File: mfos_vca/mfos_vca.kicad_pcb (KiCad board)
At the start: 2 copper layers, 196.4 x 297.5 mm, 95 parts, among them J1 CV A, J2 Signal In A, J3 Signal Out A, J4 CV B, J5 CV1 B, J5 Signal In B, J6 Signal Out B, J7 Conn_02x05_Odd_Even, Q1 2N3904, Q2 2N3906, Q3 2N3904, Q4 2N3906, SW1 SW_SPDT, SW2 SW_SPDT, U1 TL074, U2 LM13700

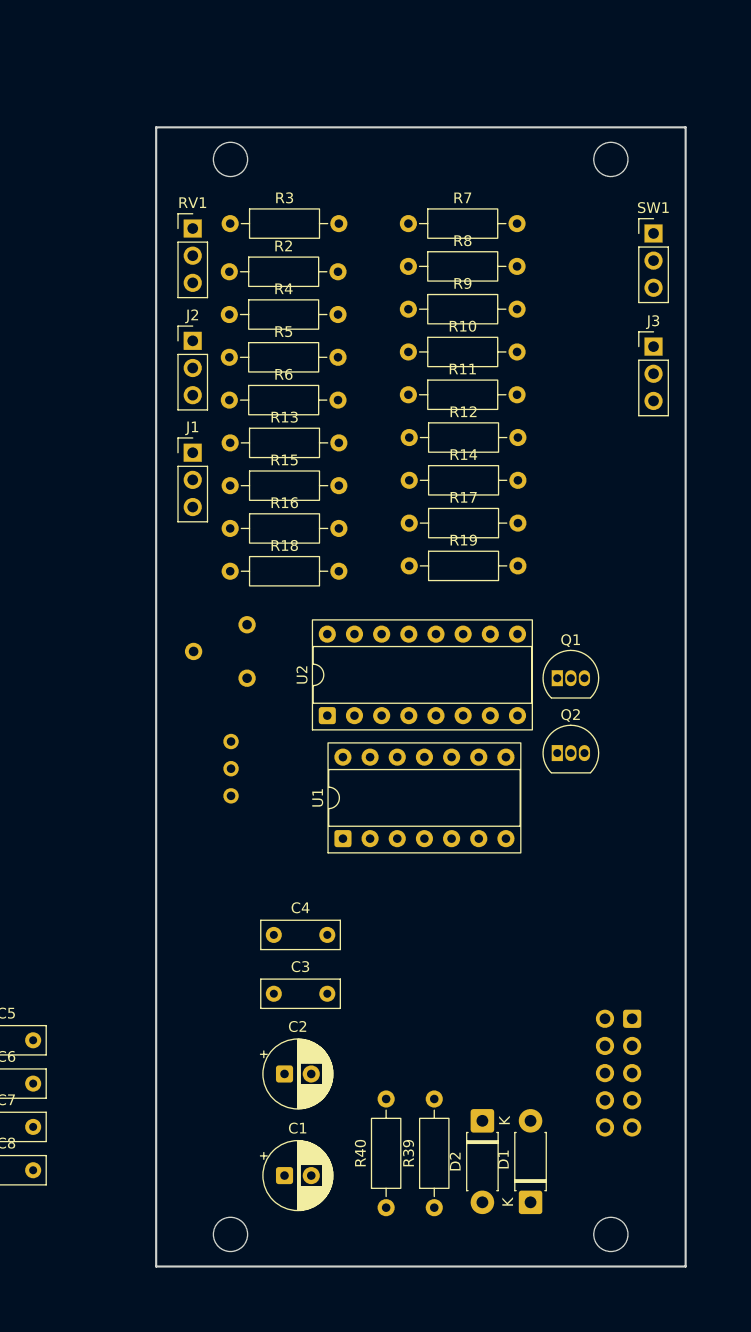
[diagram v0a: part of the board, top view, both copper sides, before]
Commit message: vca pcb progress from last night
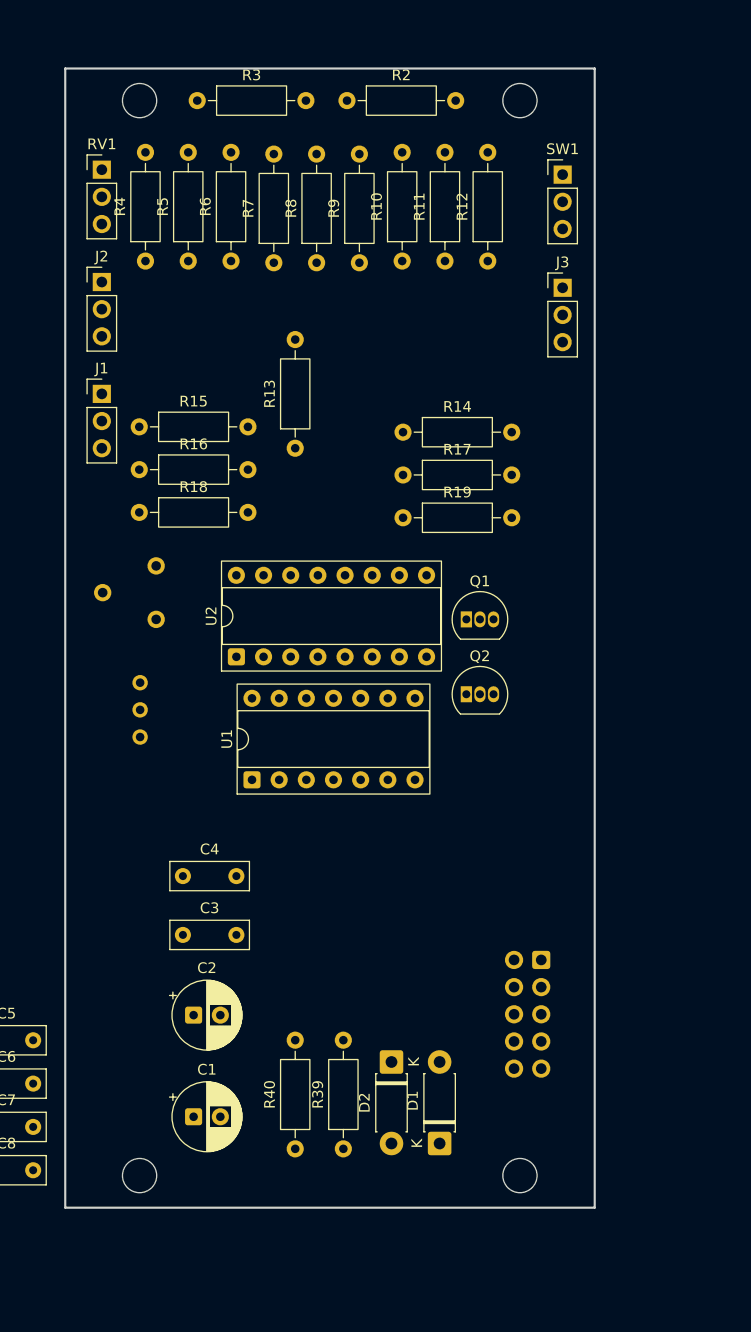
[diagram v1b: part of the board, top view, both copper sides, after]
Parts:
- moved R2 19.4 mm to (258.8, 43.5)
- moved R12 18.1 mm to (272.0, 58.5), turned to 90 degrees
- moved R7 13.1 mm to (252.0, 58.7), turned to 90 degrees
- moved R6 13.0 mm to (248.0, 58.5), turned to 90 degrees
- moved R11 13.0 mm to (268.0, 58.5), turned to 90 degrees
- moved R3 11.9 mm to (244.8, 43.5)
- moved C1 10.1 mm to (244.5, 138.5)
- moved C2 10.1 mm to (244.5, 129.0)
- moved C3 10.1 mm to (243.5, 121.5)
- moved C4 10.1 mm to (243.5, 116.0)
- moved D1 10.1 mm to (267.5, 141.0)
- moved D2 10.1 mm to (263.0, 133.4)
- moved J1 10.1 mm to (235.9, 70.9)
- moved J3 10.1 mm to (279.0, 61.0)
- moved J7 10.1 mm to (277.0, 123.8)
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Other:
- outline, holes or cut-outs redrawn
